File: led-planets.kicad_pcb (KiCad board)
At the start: 2 copper layers, 40 parts, among them J1 SM08B-GHS-TB, J2 SM08B-GHS-TB, J3 Conn_01x05, Q1 MMBT2222A, Q2 MMBT2222A, Q3 MMBT2222A, Q4 MMBT2222A, Q5 MMBT2222A, Q6 MMBT2222A, Q7 MMBT2222A, Q8 MMBT2222A, U2 ESP32 Module

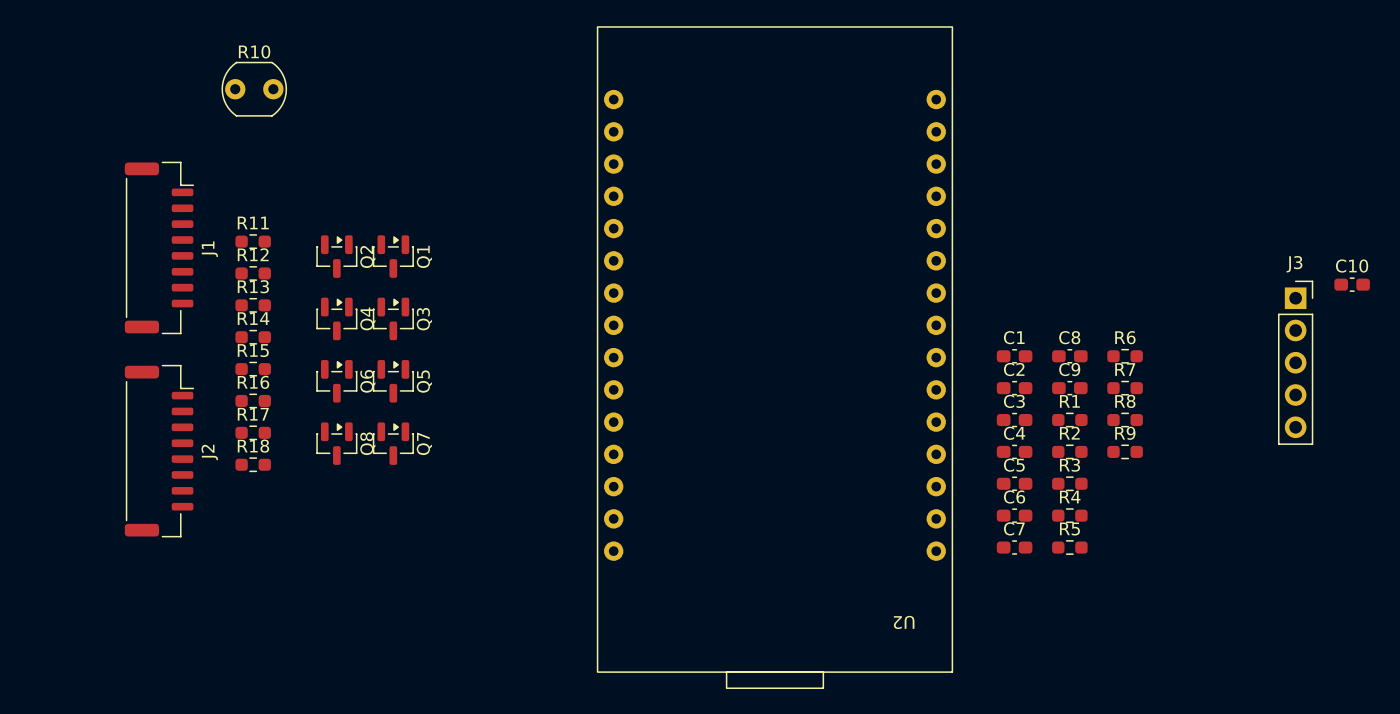
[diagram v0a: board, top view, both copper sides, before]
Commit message: layout
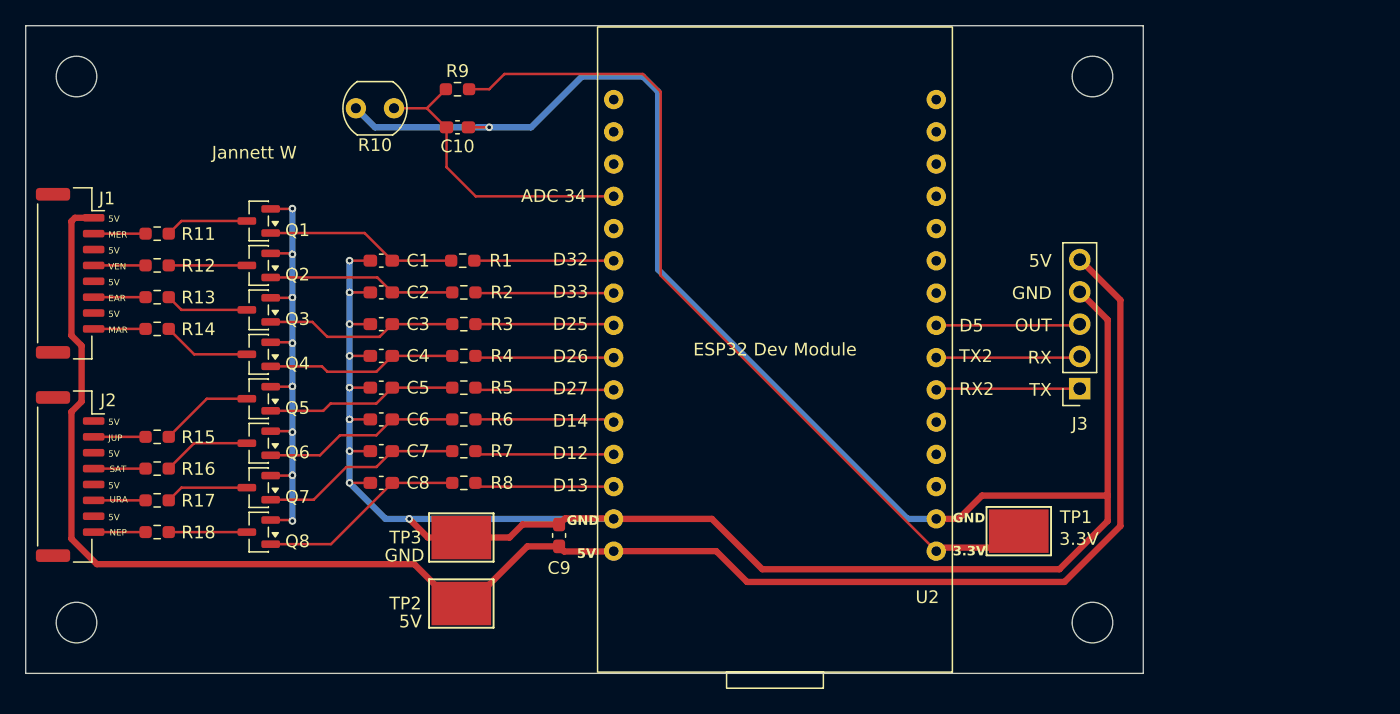
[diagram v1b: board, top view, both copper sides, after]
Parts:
- added H1: M3, MountingHole:MountingHole_3.2mm_M3, F.Cu at (50.0, 52.0)
- added H2: M3, MountingHole:MountingHole_3.2mm_M3, F.Cu at (130.0, 52.0)
- added H3: M3, MountingHole:MountingHole_3.2mm_M3, F.Cu at (50.0, 95.0)
- added H4: M3, MountingHole:MountingHole_3.2mm_M3, F.Cu at (130.0, 95.0)
- added TP1: 5016, jannett_footprints:TestPoint_Keystone_5016_Compact, F.Cu at (124.2, 87.8)
- added TP2: 5016, jannett_footprints:TestPoint_Keystone_5016_Compact, F.Cu at (80.3, 93.5)
- added TP3: 5016, jannett_footprints:TestPoint_Keystone_5016_Compact, F.Cu at (80.3, 88.3)
- moved C10 71.5 mm to (80.0, 56.0)
- moved R9 59.8 mm to (80.0, 53.0)
- moved C8 55.1 mm to (74.0, 84.0), turned to 180 degrees
- moved R6 52.3 mm to (80.5, 79.0), turned to 180 degrees
- moved R7 52.3 mm to (80.5, 81.5), turned to 180 degrees
- moved R8 52.3 mm to (80.5, 84.0), turned to 180 degrees
- moved C7 50.4 mm to (74.0, 81.5), turned to 180 degrees
- moved C6 50.4 mm to (74.0, 79.0), turned to 180 degrees
- moved C5 50.4 mm to (74.0, 76.5), turned to 180 degrees
- moved C4 50.4 mm to (74.0, 74.0), turned to 180 degrees
- moved C3 50.4 mm to (74.0, 71.5), turned to 180 degrees
- moved C2 50.4 mm to (74.0, 69.0), turned to 180 degrees
- moved C1 50.4 mm to (74.0, 66.5), turned to 180 degrees
- moved R1 49.4 mm to (80.4, 66.5), turned to 180 degrees
- moved R5 49.4 mm to (80.5, 76.5), turned to 180 degrees
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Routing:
- net GND: track 0.00 -> 256.0 mm, vias 0 -> 18
- net +5V: track 0.00 -> 139.4 mm
- net +3.3V: track 0.00 -> 68.5 mm
- net /ADC_IN_PHOTO: track 0.00 -> 24.1 mm
- net Net-(Q8-B): track 0.00 -> 16.3 mm
- net Net-(Q7-B): track 0.00 -> 15.9 mm
- net Net-(Q6-B): track 0.00 -> 15.5 mm
- net Net-(Q3-B): track 0.00 -> 15.2 mm
- net Net-(Q1-B): track 0.00 -> 15.1 mm
- net Net-(Q5-B): track 0.00 -> 15.1 mm
- net Net-(Q4-B): track 0.00 -> 15.0 mm
- net Net-(Q2-B): track 0.00 -> 14.8 mm
- net /TX: track 0.00 -> 11.3 mm
- net /RX: track 0.00 -> 11.3 mm
- net /OUT: track 0.00 -> 11.3 mm
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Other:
- board outline added: 88 x 51 mm
- board text added: "3.3V"
- board text added: "5V"
- board text added: "ADC 34"
- board text added: "D12"
- board text added: "D13"
- board text added: "D14"
- board text added: "D25"
- board text added: "D26"
- board text added: "D27"
- board text added: "D32"
- board text added: "D33"
- board text added: "D5"
- board text added: "EAR"
- board text added: "ESP32 Dev Module"
- board text added: "GND"
- board text added: "JUP"
- board text added: "Jannett W"
- board text added: "MAR"
- board text added: "MER"
- board text added: "NEP"
- board text added: "OUT"
- board text added: "RX"
- board text added: "RX2"
- board text added: "SAT"
- board text added: "TX"
- board text added: "TX2"
- board text added: "URA"
- board text added: "VEN"
